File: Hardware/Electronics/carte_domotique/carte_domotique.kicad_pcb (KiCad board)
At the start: 2 copper layers, 63.5 x 59.7 mm, 21 parts, among them J1 Conn_02x06_Odd_Even, J10 Conn_01x04, J11 Conn_01x04, J12 Conn_01x04, J13 Conn_01x02, J14 Conn_01x02, J15 Conn_01x02, J16 Conn_01x02, J17 Conn_01x02, J18 Conn_01x02, J19 Conn_01x02, J2 Raspberry_Pi_2_3, J3 Conn_01x02, J4 Conn_01x05, J5 Conn_01x05, J6 Conn_01x03, J7 Conn_01x03, J8 Conn_01x03, J9 Conn_01x03

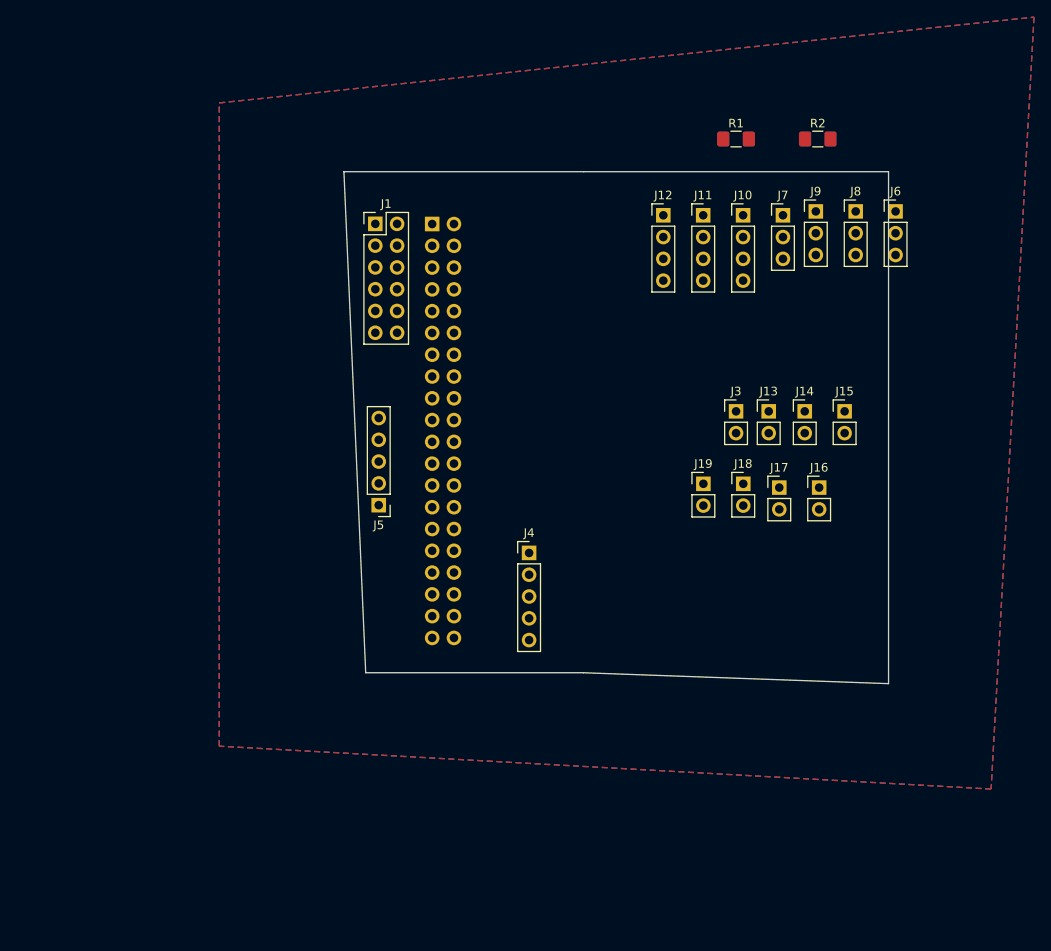
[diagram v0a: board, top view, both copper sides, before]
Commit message: carte 1
carte proto 1
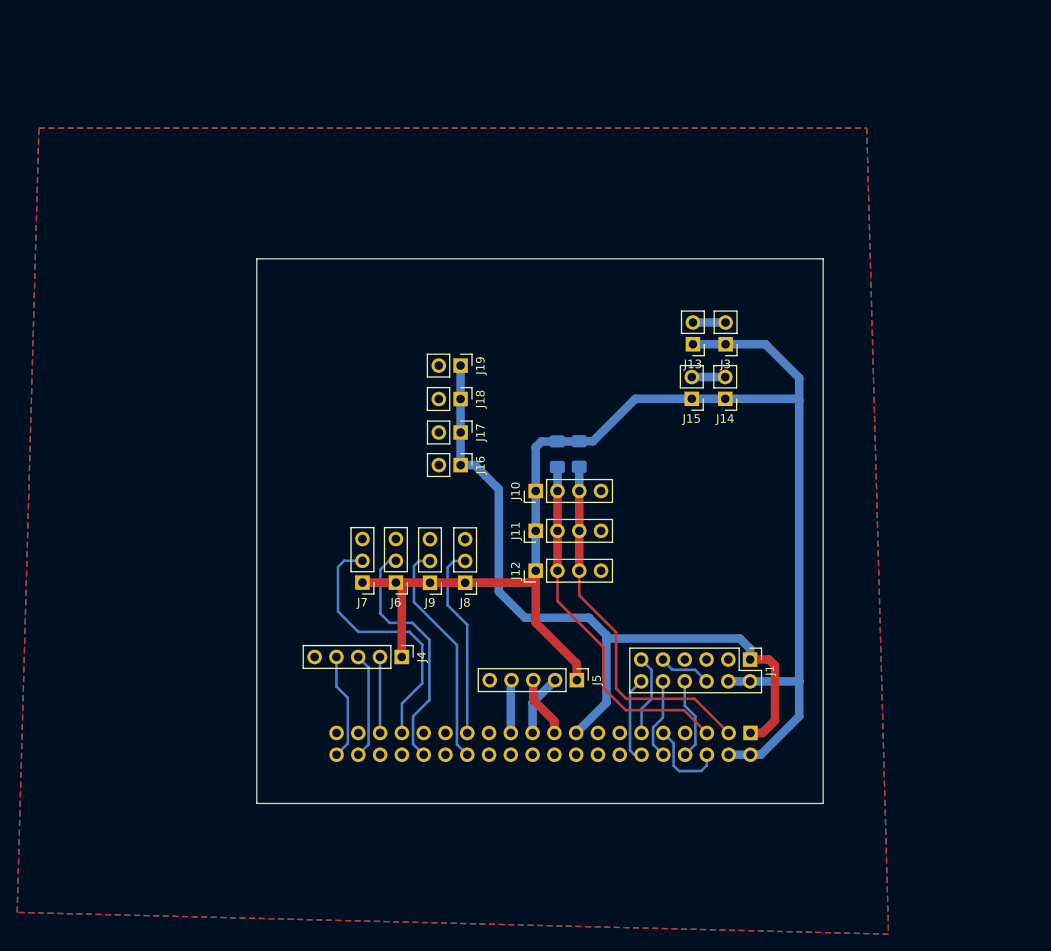
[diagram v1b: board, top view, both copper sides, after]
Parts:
- R1, R2: moved to B.Cu
- moved J6 72.6 mm to (135.6, 80.9), turned to 180 degrees
- moved J2 70.0 mm to (176.9, 98.5), turned to 90 degrees
- moved J1 67.0 mm to (176.9, 89.9), turned to 270 degrees
- moved J7 65.1 mm to (131.7, 80.9), turned to 180 degrees
- moved J8 62.8 mm to (143.7, 81.0), turned to 180 degrees
- moved J9 62.4 mm to (139.6, 81.0), turned to 180 degrees
- moved R2 46.1 mm to (157.0, 65.9), turned to 90 degrees
- moved J12 44.0 mm to (151.9, 79.5), turned to 90 degrees
- moved R1 42.2 mm to (154.4, 66.0), turned to 90 degrees
- moved J16 41.9 mm to (143.2, 67.2), turned to 270 degrees
- moved J11 41.7 mm to (151.9, 74.9), turned to 90 degrees
- moved J10 40.2 mm to (151.9, 70.2), turned to 90 degrees
- moved J17 37.7 mm to (143.2, 63.4), turned to 270 degrees
- moved J18 34.4 mm to (143.1, 59.5), turned to 270 degrees
- moved J19 31.5 mm to (143.1, 55.6), turned to 270 degrees
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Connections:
- J1 pad 2: Net-(J1-Pad2) -> +5V
- J1 pad 4: Net-(J1-Pad2) -> +5V
- J2 pad 11: Net-(J2-Pad11) -> reset
- J2 pad 2: Net-(J1-Pad2) -> +5V
- J2 pad 36: reset -> Net-(J2-Pad36)
- J2 pad 4: Net-(J1-Pad2) -> +5V
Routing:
- net +5V: track 0.00 -> 163.5 mm
- net +3V3: track 0.00 -> 88.2 mm
- net SDA: track 0.00 -> 42.9 mm
- net SCL: track 0.00 -> 42.2 mm
- net Net-(J2-Pad33): track 0.00 -> 31.0 mm
- net Net-(J2-Pad32): track 0.00 -> 29.0 mm
- net Net-(J2-Pad28): track 0.00 -> 26.7 mm
- net GND: track 0.00 -> 23.9 mm
- net Net-(J2-Pad27): track 0.00 -> 22.6 mm
- net Net-(J2-Pad40): track 0.00 -> 12.5 mm
- net Net-(J2-Pad38): track 0.00 -> 12.4 mm
- net /SW1: track 0.00 -> 10.1 mm
- net Net-(J1-Pad8): track 0.00 -> 9.57 mm
- net Net-(J1-Pad10): track 0.00 -> 9.54 mm
- net reset: track 0.00 -> 9.54 mm
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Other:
- board size 63.5 x 59.7 mm -> 66 x 63.5 mm
